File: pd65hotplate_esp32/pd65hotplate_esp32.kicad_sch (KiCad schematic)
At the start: 17 parts, among them U1 TPS54202DDCR, U2 HUSB238_002DD, U3 ESP32-S3-WROOM-1U-N16R8, U4 STUSB4500QTR, U5 HUSB238A, U6 LMR38020SDDAR

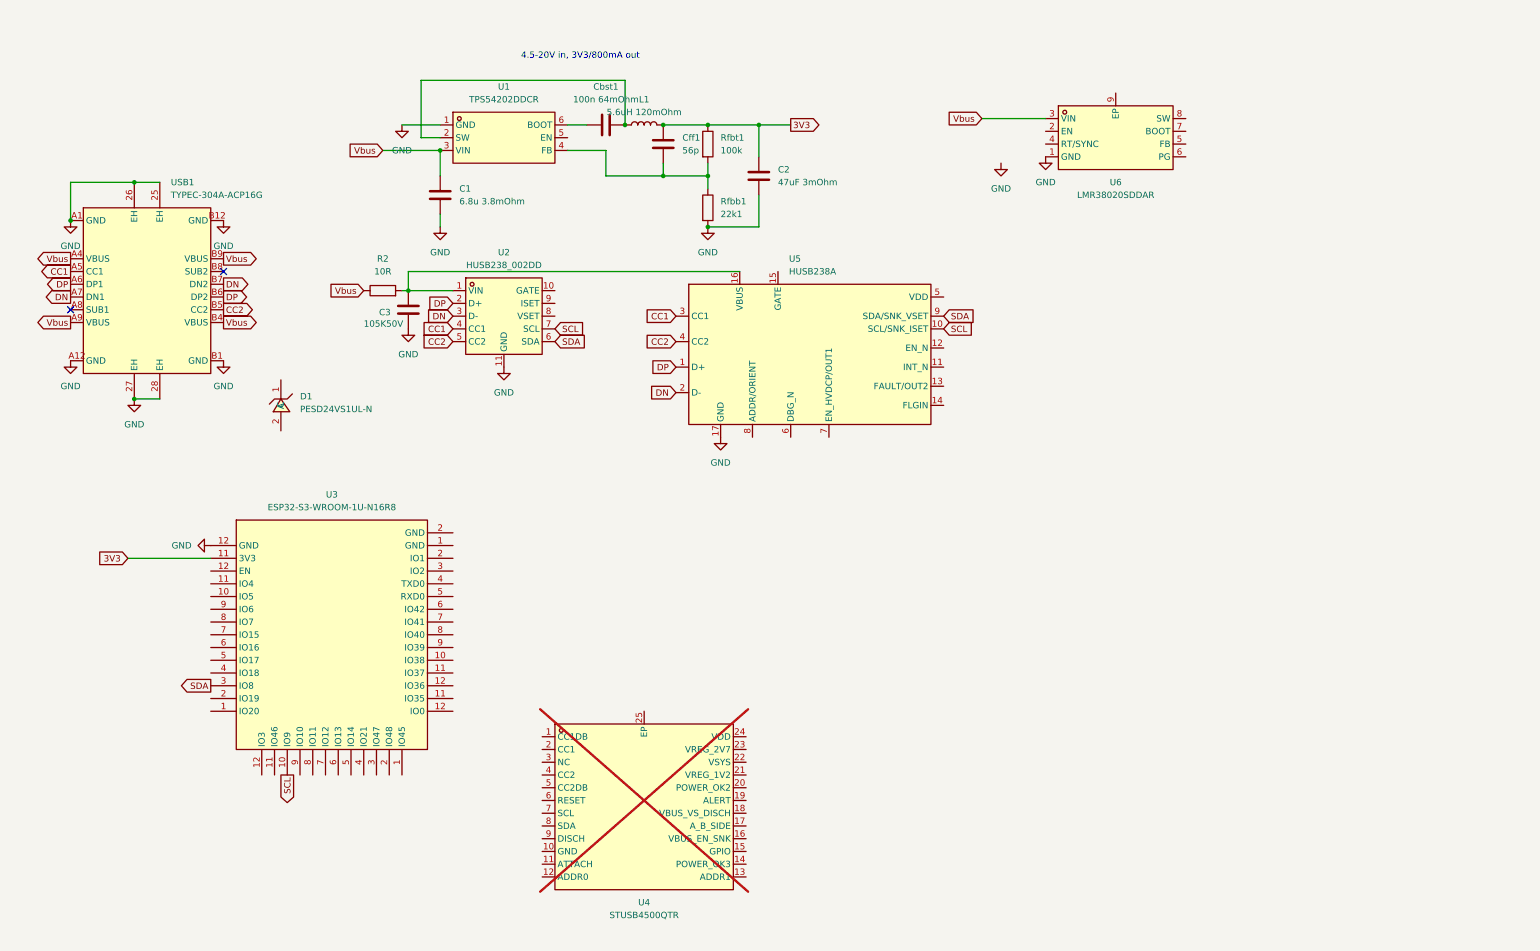
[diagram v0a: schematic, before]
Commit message: ř
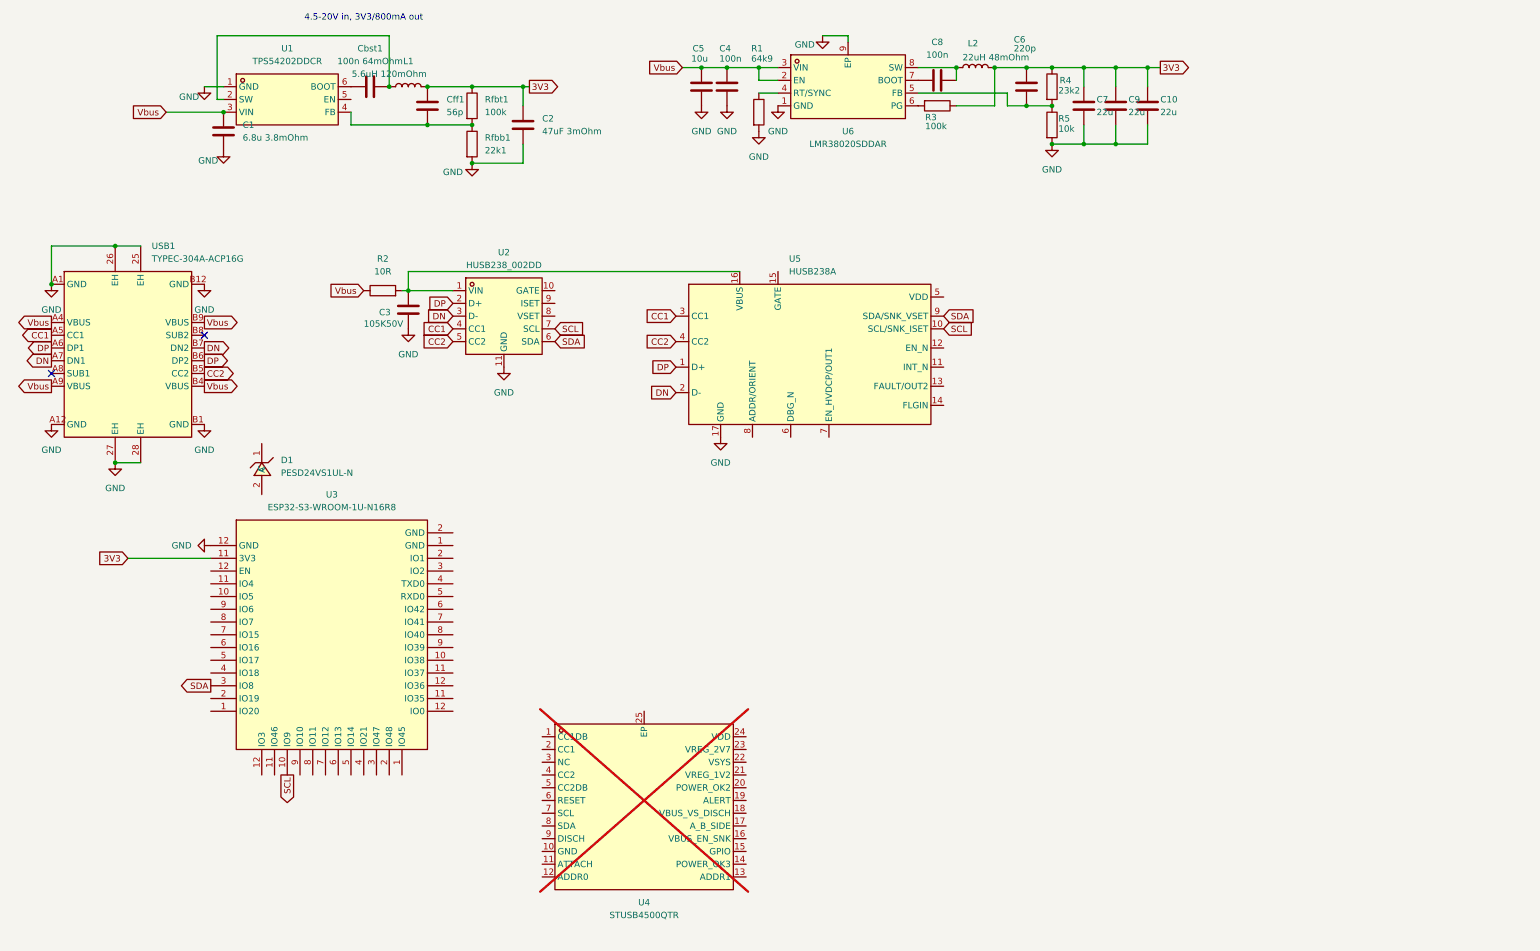
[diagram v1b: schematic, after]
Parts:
- added C10, C7, C9: 22u, symbol Device:C
- added C4, C8: 100n, symbol Device:C
- added C5: 10u, symbol Device:C
- added C6: 220p, symbol Device:C
- added L2: 22uH 48mOhm, symbol Device:L
- added R1: 64k9, symbol Device:R
- added R3: 100k, symbol Device:R
- added R4: 23k2, symbol Device:R
- added R5: 10k, symbol Device:R
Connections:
- net 3V3: now also C10.1, C6.1, C7.1, C9.1, L2.2, R3.1, R4.1
- net GND: now also U6.9 (EP), C10.2, C4.2, C5.2, C7.2, C9.2, R1.2, R5.2
- net Vbus: now also U6.2 (EN), C4.1, C5.1
- net at U6.4 (RT/SYNC): now also R1.1
- net at U6.5 (FB): now also C6.2, R4.2, R5.1
- net at U6.6 (PG): now also R3.2
- net at U6.7 (BOOT): now also C8.1
- net at U6.8 (SW): now also C8.2, L2.1
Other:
- moved on the sheet: C1, C2, Cbst1, Cff1, D1, L1, Rfbb1, Rfbt1, U1, U6, USB1

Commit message: prac
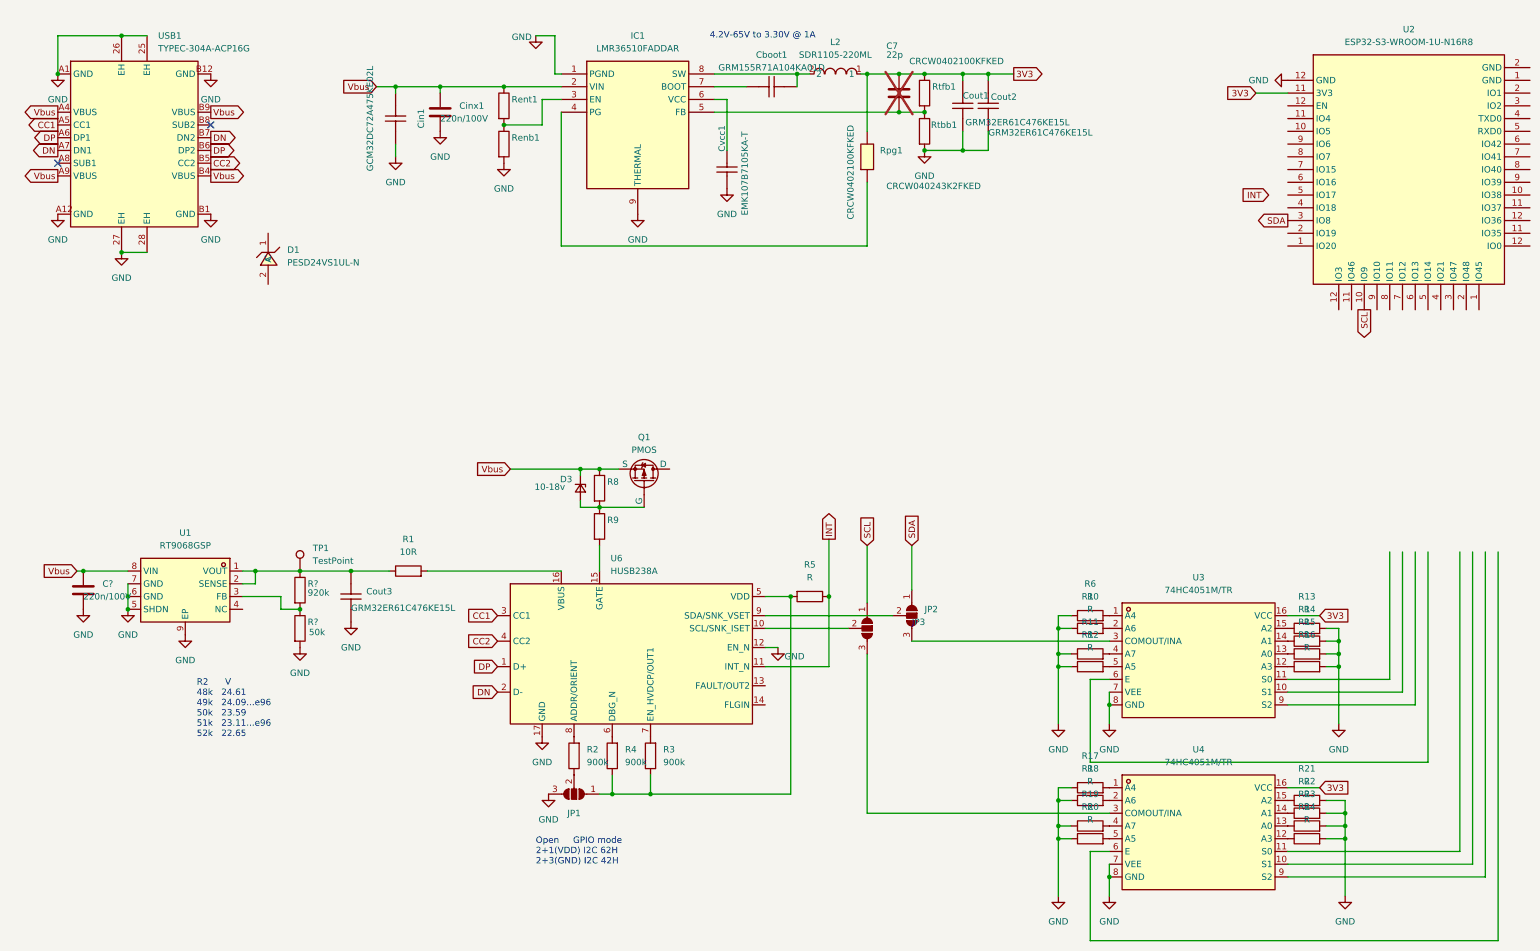
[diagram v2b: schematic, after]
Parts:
- removed C1: 6.8u 3.8mOhm, symbol Device:C
- removed C10, C9: 22u, symbol Device:C
- removed C2: 47uF 3mOhm, symbol Device:C
- removed C3: 105K50V, symbol Device:C
- removed C4, C8: 100n, symbol Device:C
- removed C5: 10u, symbol Device:C
- removed C6: 220p, symbol Device:C
- removed Cbst1: 100n 64mOhm, symbol Device:C
- removed Cff1: 56p, symbol Device:C
- removed L1: 5.6uH 120mOhm, symbol Device:L
- removed L2: 22uH 48mOhm, symbol Device:L
- removed R1: 64k9, symbol Device:R
- removed Rfbb1: 22k1, symbol Device:R
- removed Rfbt1: 100k, symbol Device:R
- removed U1: TPS54202DDCR, easyeda2kicad:SOT-23-6_L2.9-W1.6-P0.95-LS2.8-BL, symbol EasyEda2Kicad:TPS54202DDCR
- removed U2: HUSB238_002DD, easyeda2kicad:DFN-10_L3.0-W3.0-P0.50-BL-EP2.5, symbol EasyEda2Kicad:HUSB238_002DD
- removed U4: STUSB4500QTR, easyeda2kicad:QFN-24_L4.0-W4.0-P0.50-BL-EP2.8, symbol EasyEda2Kicad:STUSB4500QTR
- removed U6: LMR38020SDDAR, easyeda2kicad:ESOP-8_L4.9-W3.9-P1.27-LS6.0-BL-EP-1, symbol EasyEda2Kicad:LMR38020SDDAR
- added C?, Cinx1: 220n/100V, Capacitor_SMD:C_1206_3216Metric, symbol Device:C
- added Cboot1: GRM155R71A104KA01D, easyeda2kicad:C0402, symbol EasyEda2Kicad:GRM155R71A104KA01D
- added Cin1: GCM32DC72A475KE02L, easyeda2kicad:C1210, symbol EasyEda2Kicad:GCM32DC72A475KE02L
- added Cout1, Cout2, Cout3: GRM32ER61C476KE15L, easyeda2kicad:C1210, symbol EasyEda2Kicad:GRM32ER61C476KE15L
- added Cvcc1: EMK107B7105KA-T, easyeda2kicad:C0603, symbol EasyEda2Kicad:EMK107B7105KA-T
- added D3: 10-18v, symbol Device:D_Zener_Small
- added IC1: LMR36510FADDAR, SamacSys_Parts:SOIC127P600X170-9N, symbol SamacSys_Parts:LMR36510FADDAR
- added JP1: SolderJumper_3_Open, symbol Jumper:SolderJumper_3_Open
- added JP2, JP3: SolderJumper_3_Open, TestPoint:TestPoint_2Pads_Pitch2.54mm_Drill0.8mm, symbol Jumper:SolderJumper_3_Open
- added L2: SDR1105-220ML, easyeda2kicad:IND-SMD_L11.0-W10.0-2, symbol EasyEda2Kicad:SDR1105-220ML
- added Q1: PMOS, symbol Simulation_SPICE:PMOS
- added R10, R11, R12, R13, R14, R15, R16, R17, R18, R19, R20, R21, R22, R23, R24, R6: R, symbol Device:R
- added R2: 900k, Resistor_SMD:R_0603_1608Metric_Pad0.98x0.95mm_HandSolder, symbol Device:R
- added R8: ~, Resistor_SMD:R_0603_1608Metric_Pad0.98x0.95mm_HandSolder, symbol Device:R
- added R9: ~, easyeda2kicad:R0402, symbol Device:R
- added R?: 920k, Resistor_SMD:R_0603_1608Metric_Pad0.98x0.95mm_HandSolder, symbol Device:R
- added R?: 50k, easyeda2kicad:R0402, symbol Device:R
- added Renb1, Rtfb1: CRCW0402100KFKED, easyeda2kicad:R0402, symbol Device:R
- added Rent1: CRCW0402100KFKED, Resistor_SMD:R_0603_1608Metric_Pad0.98x0.95mm_HandSolder, symbol Device:R
- added Rpg1: CRCW0402100KFKED, easyeda2kicad:R0402, symbol EasyEda2Kicad:CRCW0402100KFKED
- added Rtbb1: CRCW040243K2FKED, easyeda2kicad:R0402, symbol Device:R
- added TP1: TestPoint, symbol Connector:TestPoint
- added U1: RT9068GSP, easyeda2kicad:ESOP-8_L4.9-W3.9-P1.27-LS6.0-BL-EP2.3, symbol EasyEda2Kicad:RT9068GSP
- added U3, U4: 74HC4051M/TR, Package_DIP:DIP-16_W7.62mm_SMDSocket_SmallPads, symbol EasyEda2Kicad:74HC4051M_TR
- C7: value 22u -> 22p; footprint (none) -> Capacitor_SMD:C_0805_2012Metric_Pad1.18x1.45mm_HandSolder; now not fitted
- R1: renamed from R2; footprint (none) -> Resistor_SMD:R_0603_1608Metric_Pad0.98x0.95mm_HandSolder
- R3: value 100k -> 900k; footprint (none) -> Resistor_SMD:R_0603_1608Metric_Pad0.98x0.95mm_HandSolder
- R4: value 23k2 -> 900k; footprint (none) -> Resistor_SMD:R_0603_1608Metric_Pad0.98x0.95mm_HandSolder
- R5: value 10k -> R
- renumbered U3 to U2, U5 to U6
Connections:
- net 3V3: now also Cout1.2, Cout2.2, L2.1, Rpg1.2, Rtfb1.1, U3.16 (VCC), U4.16 (VCC); no longer R3.1, R4.1
- net GND: now also U6.12 (EN_N), C?.2, Cin1.2, Cinx1.2, Cout1.1, Cout2.1, Cout3.1, Cvcc1.1, IC1.1 (PGND), IC1.9 (THERMAL), JP1.3 (B), R10.1, R11.1, R12.1, R13.2, R14.2, R15.2, R16.2, R17.1, R18.1, R19.1, R20.1, R21.2, R22.2, R23.2, R24.2, R6.1, R?.2, Renb1.2, Rtbb1.2, U1.5 (SHDN), U1.6 (GND), U1.7 (GND), U1.9 (EP), U3.7 (VEE), U3.8 (GND), U4.7 (VEE), U4.8 (GND); no longer C7.2, R5.2
- net SCL: now also JP3.1 (A); no longer U6.10 (SCL/SNK_ISET)
- net SDA: now also JP2.1 (A); no longer U6.9 (SDA/SNK_VSET)
- net Vbus: now also C?.1, Cin1.1, Cinx1.1, D3.1 (K), IC1.2 (VIN), Q1.3 (S), R8.1, Rent1.1, U1.8 (VIN); no longer R1.1
- net at R4.2: now also U6.6 (DBG_N); no longer R5.1
- net INT: now reaches U6.11 (INT_N)
- net INT: now also R5.1
- net at U6.15 (GATE): now also R9.2
- net at U6.5 (VDD): now also R3.1, R4.1, R5.2, JP1.1 (A)
- net at U6.7 (EN_HVDCP/OUT1): now also R3.2
- net at U6.8 (ADDR/ORIENT): now also R2.2
- new net: R21.1, U4.15 (A2)
- new net: JP2.2 (C), U6.9 (SDA/SNK_VSET)
- new net: JP2.3 (B), U3.3 (COMOUT/INA)
- new net: R14.1, U3.14 (A1)
- new net: Cout3.2, R1.1, R?.1, TP1.1, U1.1 (VOUT), U1.2 (SENSE)
- new net: R?.1, R?.2, U1.3 (FB)
- new net: Cboot1.1, IC1.8 (SW), L2.2
- new net: Cboot1.2, IC1.7 (BOOT)
- new net: R23.1, U4.13 (A0)
- new net: JP3.2 (C), U6.10 (SCL/SNK_ISET)
- new net: R19.2, U4.4 (A7)
- new net: IC1.3 (EN), Renb1.1, Rent1.2
- new net: IC1.4 (PG), Rpg1.1
- new net: C7.2, IC1.5 (FB), Rtbb1.1, Rtfb1.2
- new net: Cvcc1.2, IC1.6 (VCC)
- new net: R6.2, U3.1 (A4)
- new net: R16.1, U3.12 (A3)
- new net: R15.1, U3.13 (A0)
- new net: R13.1, U3.15 (A2)
- new net: R10.2, U3.2 (A6)
- new net: R11.2, U3.4 (A7)
- new net: R12.2, U3.5 (A5)
- new net: D3.2 (A), Q1.2 (G), R8.2, R9.1
- new net: R17.2, U4.1 (A4)
- new net: R22.1, U4.14 (A1)
- new net: JP1.2 (C), R2.1
- new net: R24.1, U4.12 (A3)
- new net: R20.2, U4.5 (A5)
- new net: R18.2, U4.2 (A6)
- new net: JP3.3 (B), U4.3 (COMOUT/INA)
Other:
- note added: "4.2V-65V to 3.30V @ 1A"
- note added: "Open GPIO mode 2+1(VDD) I2C 62H 2+3(GND) I2C 42H"
- note added: "R2 V 48k 24.61 49k 24.09...e96 50k 23.59 51k 23.11...e96 52k 22.65 ​ ​"
- note removed: "4.5-20V in, 3V3/800mA out"
- moved on the sheet: D1, R1, U2, U6, USB1
